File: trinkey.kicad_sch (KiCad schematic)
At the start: 11 parts, among them J1 USB_A, U1 STM32C071G8Ux, U2 XC6206PxxxMR

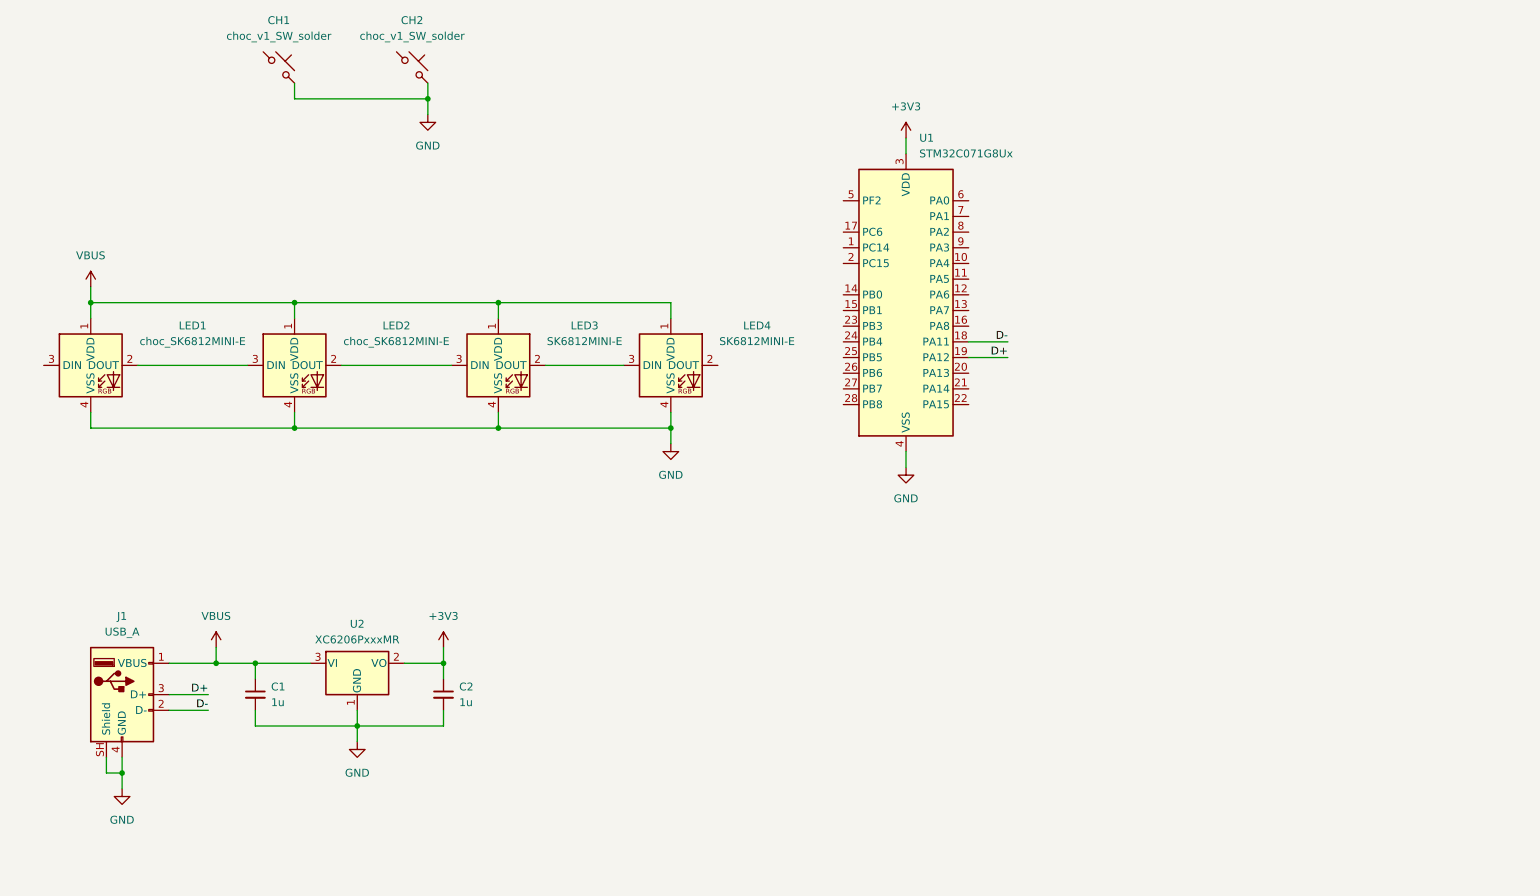
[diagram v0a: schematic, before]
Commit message: feat: polishing and readme
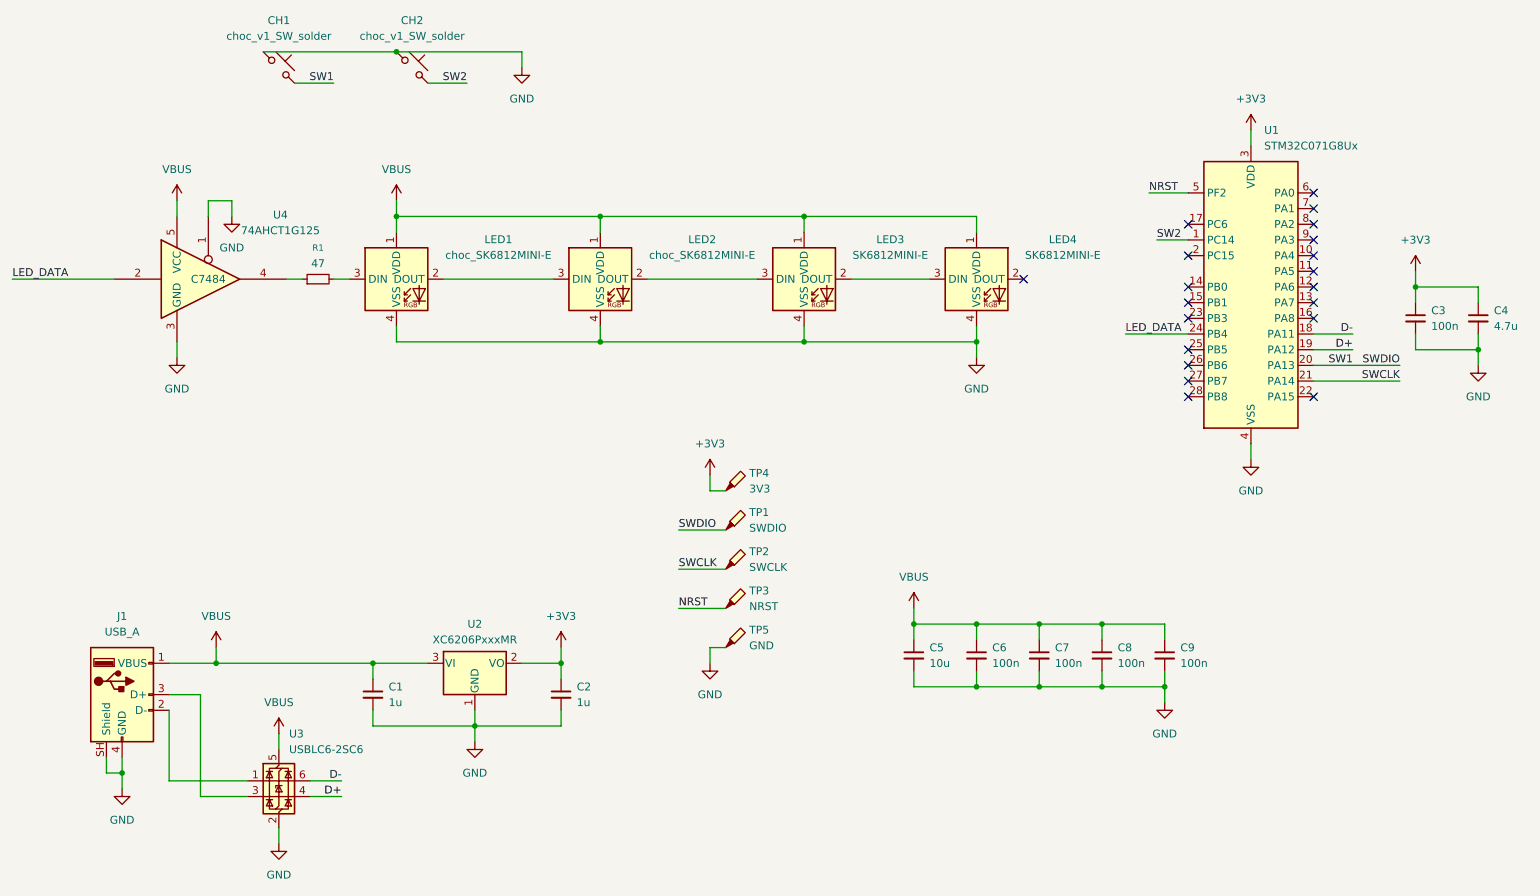
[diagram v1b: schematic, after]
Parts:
- added C3, C6, C7, C8, C9: 100n, Capacitor_SMD:C_0402_1005Metric, symbol Device:C_Small
- added C4: 4.7u, Capacitor_SMD:C_0402_1005Metric, symbol Device:C_Small
- added C5: 10u, Capacitor_SMD:C_0402_1005Metric, symbol Device:C_Small
- added R1: 47, Resistor_SMD:R_0402_1005Metric, symbol Device:R_Small
- added TP1: SWDIO, TestPoint:TestPoint_Pad_D1.0mm, symbol Connector:TestPoint_Probe
- added TP2: SWCLK, TestPoint:TestPoint_Pad_D1.0mm, symbol Connector:TestPoint_Probe
- added TP3: NRST, TestPoint:TestPoint_Pad_D1.0mm, symbol Connector:TestPoint_Probe
- added TP4: 3V3, TestPoint:TestPoint_Pad_D1.0mm, symbol Connector:TestPoint_Probe
- added TP5: GND, TestPoint:TestPoint_Pad_D1.0mm, symbol Connector:TestPoint_Probe
- added U3: USBLC6-2SC6, Package_TO_SOT_SMD:SOT-23-6, symbol Power_Protection:USBLC6-2SC6
- added U4: 74AHCT1G125, Package_TO_SOT_SMD:SOT-23-5, symbol 74xGxx:74AHCT1G125
- C1, C2: LCSC Part # (none) -> C52923
- U1: LCSC Part # (none) -> C44521811
- U2: LCSC Part # (none) -> C347376
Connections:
- net +3V3: now also C3.1, C4.1, TP4.1
- net D+: now also U3.4 (I/O2); no longer J1.3 (D+)
- net D-: now also U3.6 (I/O1); no longer J1.2 (D-)
- net GND: now also CH1.1, CH2.1, C3.2, C4.2, C5.2, C6.2, C7.2, C8.2, C9.2, TP5.1, U3.2 (GND), U4.1, U4.3 (GND); no longer CH1.2, CH2.2
- net VBUS: now also C5.1, C6.1, C7.1, C8.1, C9.1, U3.5 (VBUS), U4.5 (VCC)
- net SW2: now reaches U1.1 (PC14)
- net SW2: now also CH2.2
- net SW1: now reaches U1.20 (PA13)
- net SW1: now also CH1.2, TP1.1
- net SWCLK: now reaches U1.21 (PA14)
- net SWCLK: now also TP2.1
- net LED_DATA: now reaches U1.24 (PB4)
- net LED_DATA: now also U4.2
- net NRST: now reaches U1.5 (PF2)
- net NRST: now also TP3.1
- net at LED1.3 (DIN): now also R1.2
- new net: J1.2 (D-), U3.1 (I/O1)
- new net: J1.3 (D+), U3.3 (I/O2)
- new net: R1.1, U4.4
- no-connect marks 0 -> 20
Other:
- moved on the sheet: C1, C2, LED1, LED2, LED3, LED4, U1, U2
